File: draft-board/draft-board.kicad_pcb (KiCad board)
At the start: 4 copper layers, 55 x 70 mm, 31 parts, among them J1 24VIN, J2 24VOUT, J3 24VOUT, J4 5VOUT_GH, J5 5VOUT_XT30, K1 SLC-24VDC-SL-C, SW1 SW_SPST, U1 NB679GD-Z

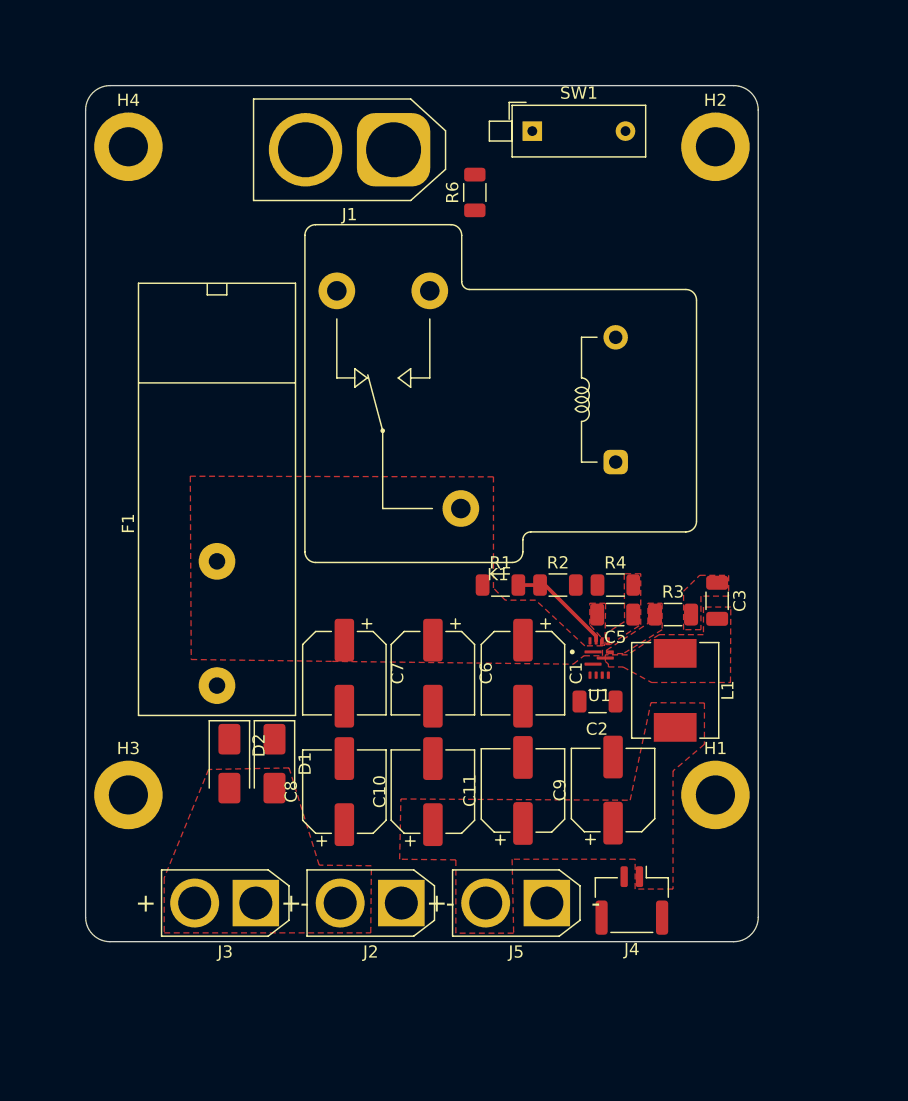
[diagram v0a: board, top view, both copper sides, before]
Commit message: Finished layout
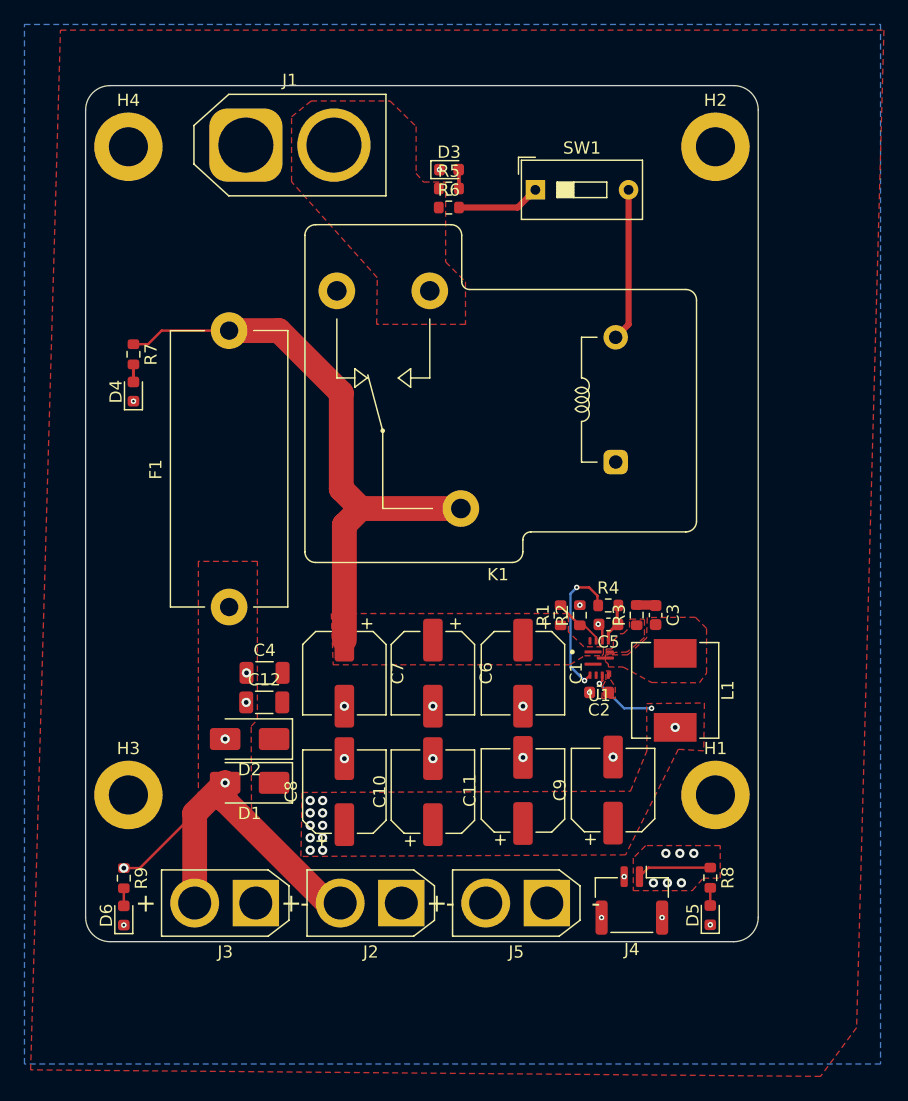
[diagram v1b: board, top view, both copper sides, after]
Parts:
- added C12: 22u, Capacitor_SMD:C_1206_3216Metric, F.Cu at (114.6, 100.4)
- added C4: 22u, Capacitor_SMD:C_1206_3216Metric, F.Cu at (114.6, 98.0)
- added D3: LED, LED_SMD:LED_0603_1608Metric, F.Cu at (129.7, 56.9)
- added D4: LED, LED_SMD:LED_0603_1608Metric, F.Cu at (103.9, 75.0)
- added D5: LED, LED_SMD:LED_0603_1608Metric, F.Cu at (151.1, 117.8)
- added D6: LED, LED_SMD:LED_0603_1608Metric, F.Cu at (103.1, 117.9)
- added R5: 100k, Resistor_SMD:R_0603_1608Metric, F.Cu at (129.7, 58.4)
- added R7: 100k, Resistor_SMD:R_0603_1608Metric, F.Cu at (103.9, 72.0)
- added R8: 100k, Resistor_SMD:R_0603_1608Metric, F.Cu at (151.1, 114.8)
- added R9: 100k, Resistor_SMD:R_0603_1608Metric, F.Cu at (103.1, 114.8)
- C2, C3, C5: footprint Capacitor_SMD:C_1206_3216Metric -> Capacitor_SMD:C_0603_1608Metric
- F1: footprint Fuse:Fuseholder_Cylinder-5x20mm_Bulgin_FX0457_Horizontal_Closed -> Fuse:Fuseholder_Cylinder-5x20mm_Stelvio-Kontek_PTF78_Horizontal_Open
- R1, R2, R4, R6: footprint Resistor_SMD:R_1206_3216Metric -> Resistor_SMD:R_0603_1608Metric
- R3: footprint Capacitor_SMD:C_1206_3216Metric -> Resistor_SMD:R_0603_1608Metric
- SW1: footprint Button_Switch_THT:SW_DIP_SPSTx01_Piano_10.8x4.1mm_W7.62mm_P2.54mm -> Button_Switch_THT:SW_DIP_SPSTx01_Slide_9.78x4.72mm_W7.62mm_P2.54mm
- moved J1 12.1 mm to (113.1, 54.9), turned to 0 degrees
- moved F1 6.50 mm to (111.7, 92.6)
- moved R1 5.50 mm to (138.8, 93.3), turned to 90 degrees
- moved C3 5.16 mm to (146.6, 93.3)
- moved SW1 4.81 mm to (136.8, 58.5)
- moved R2 3.05 mm to (140.4, 93.3), turned to 90 degrees
- moved R3 2.97 mm to (145.1, 93.3), turned to 90 degrees
- moved D2 2.60 mm to (113.4, 103.4), turned to 180 degrees
- moved D1 2.57 mm to (113.4, 107.0), turned to 180 degrees
- moved R6 2.45 mm to (129.7, 60.0), turned to 0 degrees
- moved R4 1.77 mm to (142.7, 92.5)
- moved C5 0.98 mm to (142.7, 94.1)
- moved C2 0.75 mm to (142.0, 99.6)
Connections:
- D1 pad 1: Net-(D1-A1) -> GND
- D2 pad 1: Net-(D1-A1) -> GND
- F1 pad 1: Net-(D1-A1) -> 24VOUT
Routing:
- net +24V: track 0.00 -> 49.2 mm
- net 24VOUT: track 0.00 -> 32.8 mm, vias 0 -> 5
- net Net-(SW1-B): track 0.00 -> 12.5 mm
- net +5V: track 0.00 -> 12.0 mm, vias 0 -> 19
- net Net-(U1-PG): track 0.00 -> 11.7 mm, vias 0 -> 2
- net Net-(SW1-A): track 0.00 -> 6.85 mm
- net Net-(U1-EN): track 8.48 -> 4.72 mm
- net Net-(U1-VCC): track 0.00 -> 3.23 mm
- net Net-(C3-Pad1): track 0.00 -> 1.57 mm
- net Net-(D3-A): track 0.00 -> 1.56 mm
- net GND: track 0.00 -> 1.51 mm, vias 0 -> 17
- net Net-(D5-A): track 0.00 -> 1.45 mm
- net Net-(D6-A): track 0.00 -> 1.44 mm
- net Net-(D4-A): track 0.00 -> 1.44 mm
- added copper zone on In1.Cu, net +24V
- added copper zone on In1.Cu, net +5V
- added copper zone on F.Cu, net 24VDC
- added copper zone on In1.Cu, net 24VDC
- added copper zone on In1.Cu, net 24VOUT
- added copper zone on B.Cu, net GND
- added copper zone on In2.Cu, net GND
- added copper zone on F.Cu, net Net-(U1-LDO)
- removed copper zone on F.Cu, net Net-(C3-Pad1)
- removed copper zone on F.Cu, net Net-(U1-VCC)
